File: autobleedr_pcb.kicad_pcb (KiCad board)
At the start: 4 copper layers, 88.6 x 91 mm, 30 parts, among them J1 Barrel_Jack, J10 XT60 Connector, J11 Conn_01x02_Pin, J13 Screw_Terminal_01x08, J2 Conn_01x01_Pin, J4 Conn_01x13_Pin, J5 Conn_01x13_Pin, J7 Screw_Terminal_01x02, J8 Conn_01x02_Pin, J9 Conn_01x02_Pin, U2 ESP32, U4 Buck Converter, U6 TMC2209

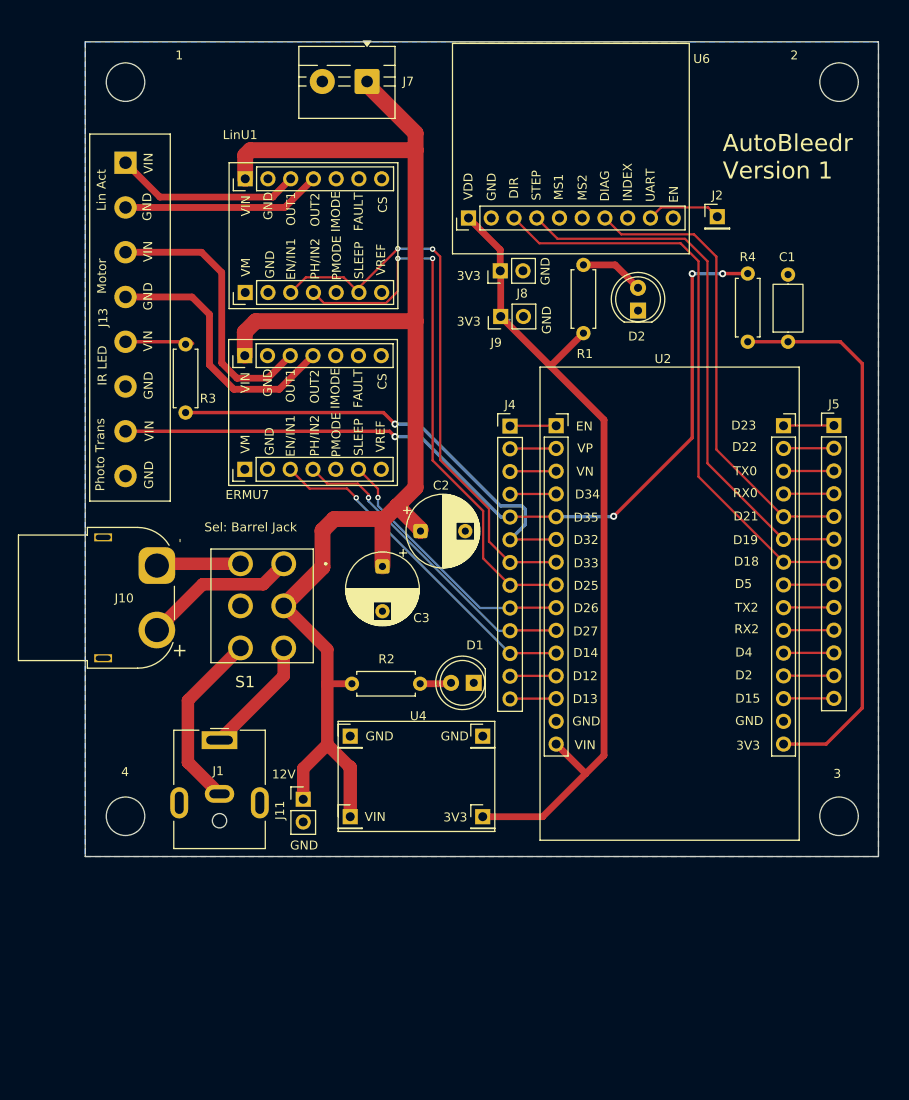
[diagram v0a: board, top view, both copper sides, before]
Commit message: updated v2
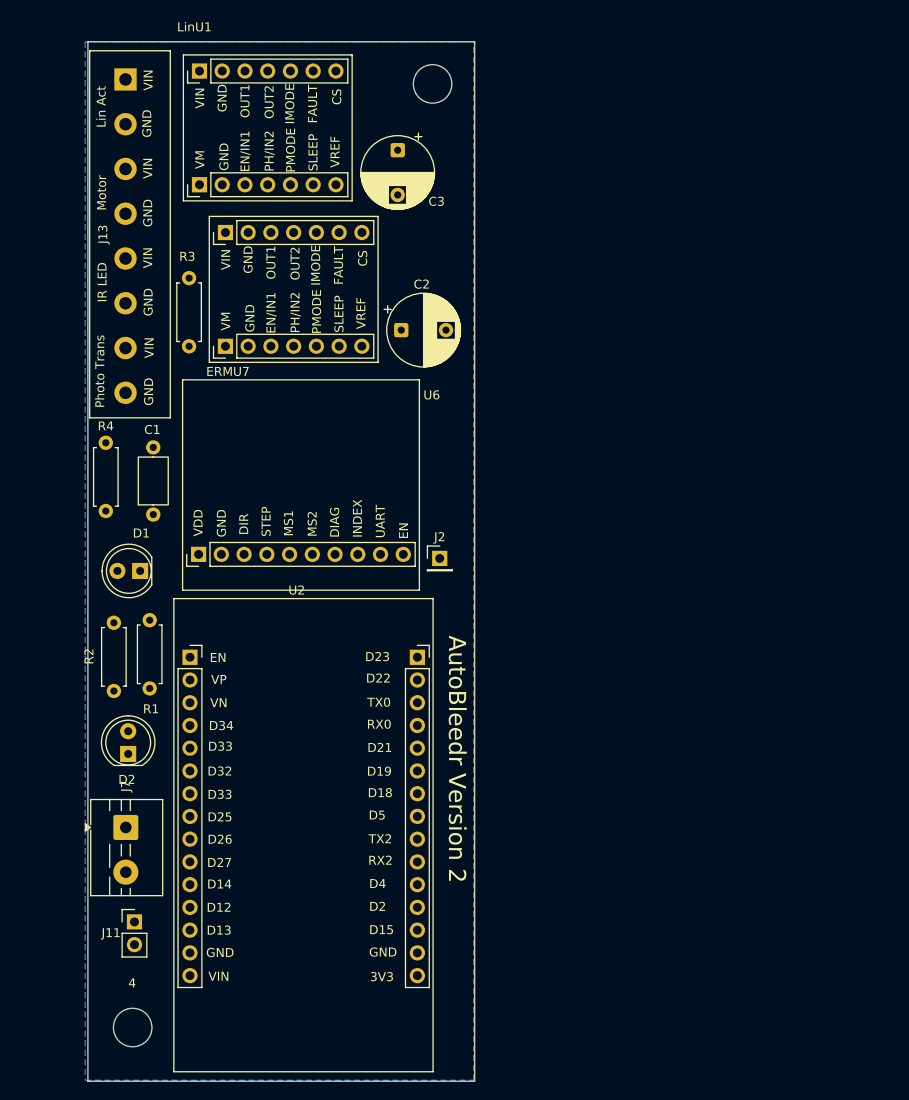
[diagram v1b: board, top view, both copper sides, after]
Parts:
- removed 1, 3: MountingHole_4.3mm_M4_ISO7380_Pad, MountingHole:MountingHole_4.3mm_M4_ISO7380_Pad
- removed J1: Barrel_Jack, Connector_BarrelJack:BarrelJack_CUI_PJ-063AH_Horizontal
- removed J10: XT60 Connector, Connector_AMASS:AMASS_XT60PW-F_1x02_P7.20mm_Horizontal
- removed J4, J5: Conn_01x13_Pin, Connector_PinHeader_2.54mm:PinHeader_1x13_P2.54mm_Vertical
- removed J8, J9: Conn_01x02_Pin, Connector_PinHeader_2.54mm:PinHeader_1x02_P2.54mm_Vertical
- removed S1: 7201SYCQE, Capstone_Footprints:7201SYCQE
- removed U4: Buck Converter, Capstone_Footprints:Buck_Converter
- moved J7 87.6 mm to (53.5, 148.7), turned to -90 degrees
- moved D2 75.5 mm to (53.8, 140.5)
- moved R4 74.2 mm to (51.3, 113.4)
- moved C1 73.5 mm to (56.6, 113.8)
- moved R1 62.6 mm to (56.2, 125.6)
- moved J2 49.2 mm to (88.6, 118.7)
- moved U2 48.4 mm to (60.8, 129.7)
- moved U6 48.2 mm to (73.0, 110.7)
- moved C3 46.5 mm to (83.9, 73.1)
- moved 2 45.4 mm to (87.8, 65.7)
- moved D1 39.3 mm to (55.1, 120.1)
- moved R2 34.9 mm to (52.2, 125.9), turned to -90 degrees
- moved 4 23.6 mm to (54.3, 171.1)
- moved J11 23.3 mm to (54.5, 159.3)
- moved C2 22.6 mm to (84.3, 93.2)
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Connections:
- C1 pad 1: 3V3 -> +3.3V
- C2 pad 1: +12V -> +7.4V
- C3 pad 1: +12V -> +7.4V
- ERMU7 pad 14: +12V -> +7.4V
- J11 pad 1: +12V -> +7.4V
- J7 pad 1: +12V -> +7.4V
- LinU1 pad 14: +12V -> +7.4V
- R2 pad 2: +12V -> +7.4V
- R4 pad 1: 3V3 -> +3.3V
- U2 pad 1: Net-(J4-Pin_1) -> unconnected-(U2-EN-Pad1)
- U2 pad 12: Net-(J4-Pin_12) -> unconnected-(U2-D12-Pad12)
- U2 pad 13: Net-(J4-Pin_13) -> unconnected-(U2-D13-Pad13)
- U2 pad 15: +3.3V -> +7.4V
- U2 pad 16: 3V3 -> +3.3V
- U2 pad 18: Net-(J5-Pin_13) -> unconnected-(U2-D15-Pad18)
- U2 pad 19: Net-(J5-Pin_12) -> unconnected-(U2-D2-Pad19)
- U2 pad 2: Net-(J4-Pin_2) -> unconnected-(U2-VP-Pad2)
- U2 pad 20: Net-(J5-Pin_11) -> unconnected-(U2-D4-Pad20)
- U2 pad 21: Net-(J5-Pin_10) -> unconnected-(U2-RX2-Pad21)
- U2 pad 22: Net-(J5-Pin_9) -> unconnected-(U2-TX2-Pad22)
- U2 pad 23: Net-(J5-Pin_8) -> unconnected-(U2-D5-Pad23)
- U2 pad 27: Net-(J5-Pin_4) -> unconnected-(U2-RX0-Pad27)
- U2 pad 28: Net-(J5-Pin_3) -> unconnected-(U2-TX0-Pad28)
- U2 pad 29: Net-(J5-Pin_2) -> unconnected-(U2-D22-Pad29)
- U2 pad 3: Net-(J4-Pin_3) -> unconnected-(U2-VN-Pad3)
- U2 pad 30: Net-(J5-Pin_1) -> unconnected-(U2-D23-Pad30)
- U2 pad 4: Net-(J4-Pin_4) -> unconnected-(U2-D34-Pad4)
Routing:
- net +12V: track 160.8 -> 0.00 mm
- net D35: track 95.4 -> 0.00 mm, vias 4 -> 0
- net +3.3V: track 92.7 -> 0.00 mm
- net /DIR: track 65.8 -> 0.00 mm
- net /enable DRV: track 63.3 -> 0.00 mm, vias 2 -> 0
- net /linear actuator direction: track 63.2 -> 0.00 mm, vias 2 -> 0
- net 3V3: track 62.7 -> 0.00 mm
- net /STEP: track 61.3 -> 0.00 mm
- net /DIAG: track 52.0 -> 0.00 mm
- net D32: track 51.6 -> 0.00 mm, vias 1 -> 0
- net /speed ERM DRV: track 38.3 -> 0.00 mm, vias 1 -> 0
- net /direction ERM DRV: track 35.0 -> 0.00 mm, vias 1 -> 0
- net /ERM vin: track 31.2 -> 0.00 mm
- net /ERM gnd: track 30.1 -> 0.00 mm
- net /enable ERM DRV: track 29.6 -> 0.00 mm, vias 1 -> 0
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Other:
- board size 88.6 x 91 mm -> 43.2 x 116.1 mm
- board text added: "AutoBleedr Version 2"
- board text added: "D33"
- board text removed: "12V"
- board text removed: "3V3"
- board text removed: "AutoBleedr Version 1"
- board text removed: "GND"
- board text removed: "Sel: Barrel Jack"
